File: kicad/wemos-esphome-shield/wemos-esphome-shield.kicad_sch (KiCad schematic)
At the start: 27 parts, among them Q1 2N2219, Q2 2N2219, Q3 2N2219, T1 Transformer_1P_1S, U1 WeMos_D1_mini

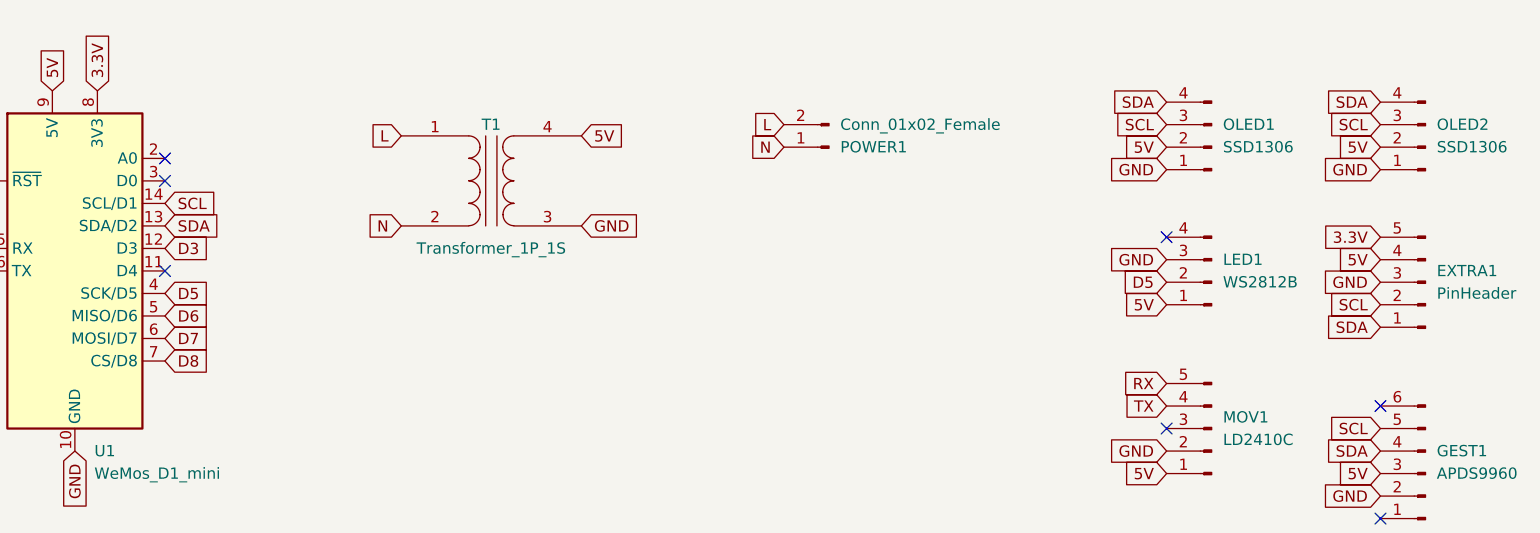
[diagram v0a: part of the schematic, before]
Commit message: wire tracks
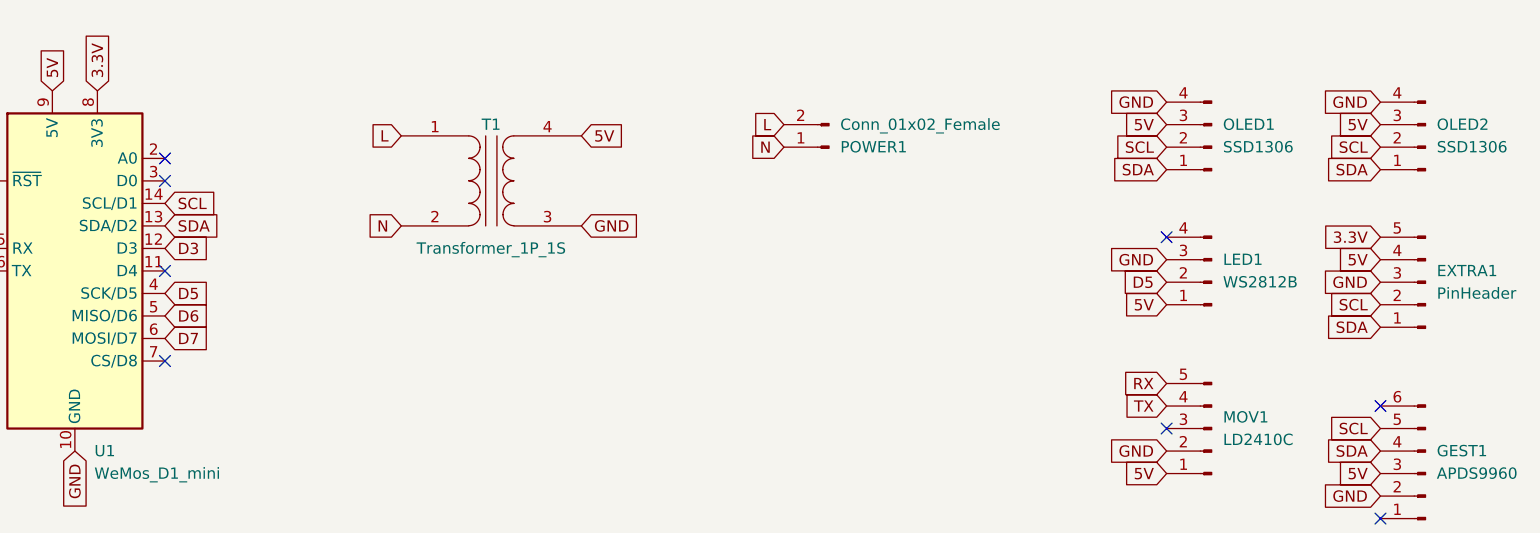
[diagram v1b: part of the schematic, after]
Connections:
- net 5V: now also OLED1.3 (Pin_3), OLED2.3 (Pin_3); no longer OLED1.2 (Pin_2), OLED2.2 (Pin_2)
- net GND: now also OLED1.4 (Pin_4), OLED2.4 (Pin_4); no longer OLED1.1 (Pin_1), OLED2.1 (Pin_1)
- net SCL: now also OLED1.2 (Pin_2), OLED2.2 (Pin_2); no longer OLED1.3 (Pin_3), OLED2.3 (Pin_3)
- net SDA: now also OLED1.1 (Pin_1), OLED2.1 (Pin_1); no longer OLED1.4 (Pin_4), OLED2.4 (Pin_4)
- net D8: no longer names the net of U1.7 (CS/D8)
- no-connect marks 9 -> 10
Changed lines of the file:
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@@
   (no_connect (at 55.88 40.64))
   (no_connect (at 55.88 30.48))
+  (no_connect (at 55.88 50.8))
   (no_connect (at 193.04 68.58))
   (no_connect (at 193.04 55.88))
@@
     )
   )
-  (global_label "D8" (shape input) (at 55.88 50.8 0) (fields_autoplaced)
-    (effects (font (size 1.27 1.27)) (justify left))
-    (property "Intersheetrefs" "${INTERSHEET_REFS}" (at 61.3447 50.8 0)
-      (effects (font (size 1.27 1.27)) (justify left) hide)
-    )
-  )
-  (global_label "SCL" (shape input) (at 193.04 24.13 180) (fields_autoplaced)
-    (effects (font (size 1.27 1.27)) (justify right))
-    (property "Intersheetrefs" "${INTERSHEET_REFS}" (at 187.1193 24.2094 0)
+  (global_label "SCL" (shape input) (at 193.04 26.67 180) (fields_autoplaced)
+    (effects (font (size 1.27 1.27)) (justify right))
+    (property "Intersheetrefs" "${INTERSHEET_REFS}" (at 187.1193 26.7494 0)
       (effects (font (size 1.27 1.27)) (justify right) hide)
     )
@@
     )
   )
-  (global_label "5V" (shape input) (at 193.04 26.67 180) (fields_autoplaced)
-    (effects (font (size 1.27 1.27)) (justify right))
-    (property "Intersheetrefs" "${INTERSHEET_REFS}" (at 188.3288 26.5906 0)
-      (effects (font (size 1.27 1.27)) (justify right) hide)
-    )
-  )
-  (global_label "SDA" (shape input) (at 168.91 21.59 180) (fields_autoplaced)
-    (effects (font (size 1.27 1.27)) (justify right))
-    (property "Intersheetrefs" "${INTERSHEET_REFS}" (at 162.9288 21.6694 0)
+  (global_label "5V" (shape input) (at 193.04 24.13 180) (fields_autoplaced)
+    (effects (font (size 1.27 1.27)) (justify right))
+    (property "Intersheetrefs" "${INTERSHEET_REFS}" (at 188.3288 24.0506 0)
+      (effects (font (size 1.27 1.27)) (justify right) hide)
+    )
+  )
+  (global_label "SDA" (shape input) (at 168.91 29.21 180) (fields_autoplaced)
+    (effects (font (size 1.27 1.27)) (justify right))
+    (property "Intersheetrefs" "${INTERSHEET_REFS}" (at 162.9288 29.2894 0)
       (effects (font (size 1.27 1.27)) (justify right) hide)
     )
@@
     )
   )
-  (global_label "GND" (shape input) (at 193.04 29.21 180) (fields_autoplaced)
-    (effects (font (size 1.27 1.27)) (justify right))
-    (property "Intersheetrefs" "${INTERSHEET_REFS}" (at 186.7564 29.1306 0)
+  (global_label "GND" (shape input) (at 193.04 21.59 180) (fields_autoplaced)
+    (effects (font (size 1.27 1.27)) (justify right))
+    (property "Intersheetrefs" "${INTERSHEET_REFS}" (at 186.7564 21.5106 0)
       (effects (font (size 1.27 1.27)) (justify right) hide)
     )
@@
     )
   )
-  (global_label "SDA" (shape input) (at 193.04 21.59 180) (fields_autoplaced)
-    (effects (font (size 1.27 1.27)) (justify right))
-    (property "Intersheetrefs" "${INTERSHEET_REFS}" (at 187.0588 21.6694 0)
+  (global_label "SDA" (shape input) (at 193.04 29.21 180) (fields_autoplaced)
+    (effects (font (size 1.27 1.27)) (justify right))
+    (property "Intersheetrefs" "${INTERSHEET_REFS}" (at 187.0588 29.2894 0)
       (effects (font (size 1.27 1.27)) (justify right) hide)
     )
@@
     )
   )
-  (global_label "GND" (shape input) (at 168.91 29.21 180) (fields_autoplaced)
-    (effects (font (size 1.27 1.27)) (justify right))
-    (property "Intersheetrefs" "${INTERSHEET_REFS}" (at 162.6264 29.1306 0)
+  (global_label "GND" (shape input) (at 168.91 21.59 180) (fields_autoplaced)
+    (effects (font (size 1.27 1.27)) (justify right))
+    (property "Intersheetrefs" "${INTERSHEET_REFS}" (at 162.6264 21.5106 0)
       (effects (font (size 1.27 1.27)) (justify right) hide)
     )
@@
     )
   )
-  (global_label "5V" (shape input) (at 168.91 26.67 180) (fields_autoplaced)
-    (effects (font (size 1.27 1.27)) (justify right))
-    (property "Intersheetrefs" "${INTERSHEET_REFS}" (at 164.1988 26.5906 0)
-      (effects (font (size 1.27 1.27)) (justify right) hide)
-    )
-  )
-  (global_label "SCL" (shape input) (at 168.91 24.13 180) (fields_autoplaced)
-    (effects (font (size 1.27 1.27)) (justify right))
-    (property "Intersheetrefs" "${INTERSHEET_REFS}" (at 162.9893 24.2094 0)
-      (effects (font (size 1.27 1.27)) (justify right) hide)
-    )
+  (global_label "5V" (shape input) (at 168.91 24.13 180) (fields_autoplaced)
+    (effects (font (size 1.27 1.27)) (justify right))
+    (property "Intersheetrefs" "${INTERSHEET_REFS}" (at 164.1988 24.0506 0)
+      (effects (font (size 1.27 1.27)) (justify right) hide)
+    )
+  )
+  (global_label "SCL" (shape input) (at 168.91 26.67 180) (fields_autoplaced)
+    (effects (font (size 1.27 1.27)) (justify right))
+    (property "Intersheetrefs" "${INTERSHEET_REFS}" (at 162.9893 26.7494 0)
+      (effects (font (size 1.27 1.27)) (justify right) hide)
+    )
